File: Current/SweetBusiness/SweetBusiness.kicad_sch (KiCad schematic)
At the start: 42 parts, among them J0 USB, J2 I2C, U0 STM32F411RETx, U1 LDO-3.3, Y1 8MHz

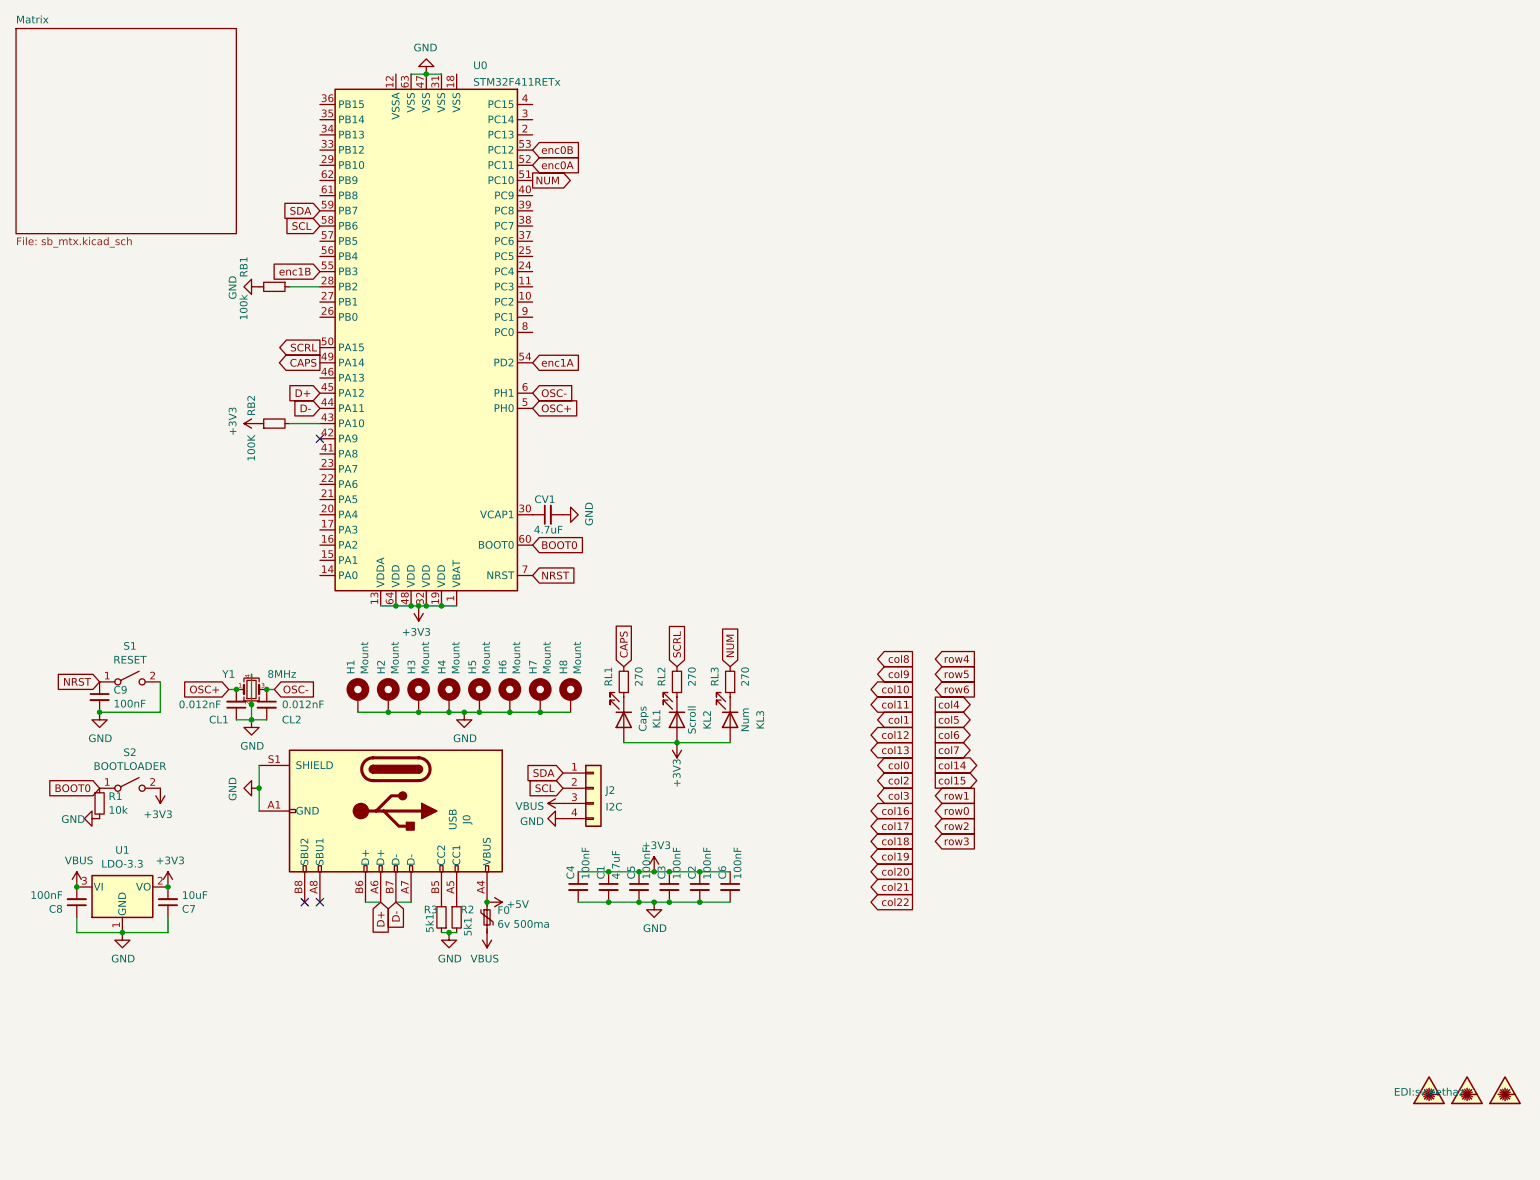
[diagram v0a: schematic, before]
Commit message: Hard Light Micro 5, Borealis, 2T, SB
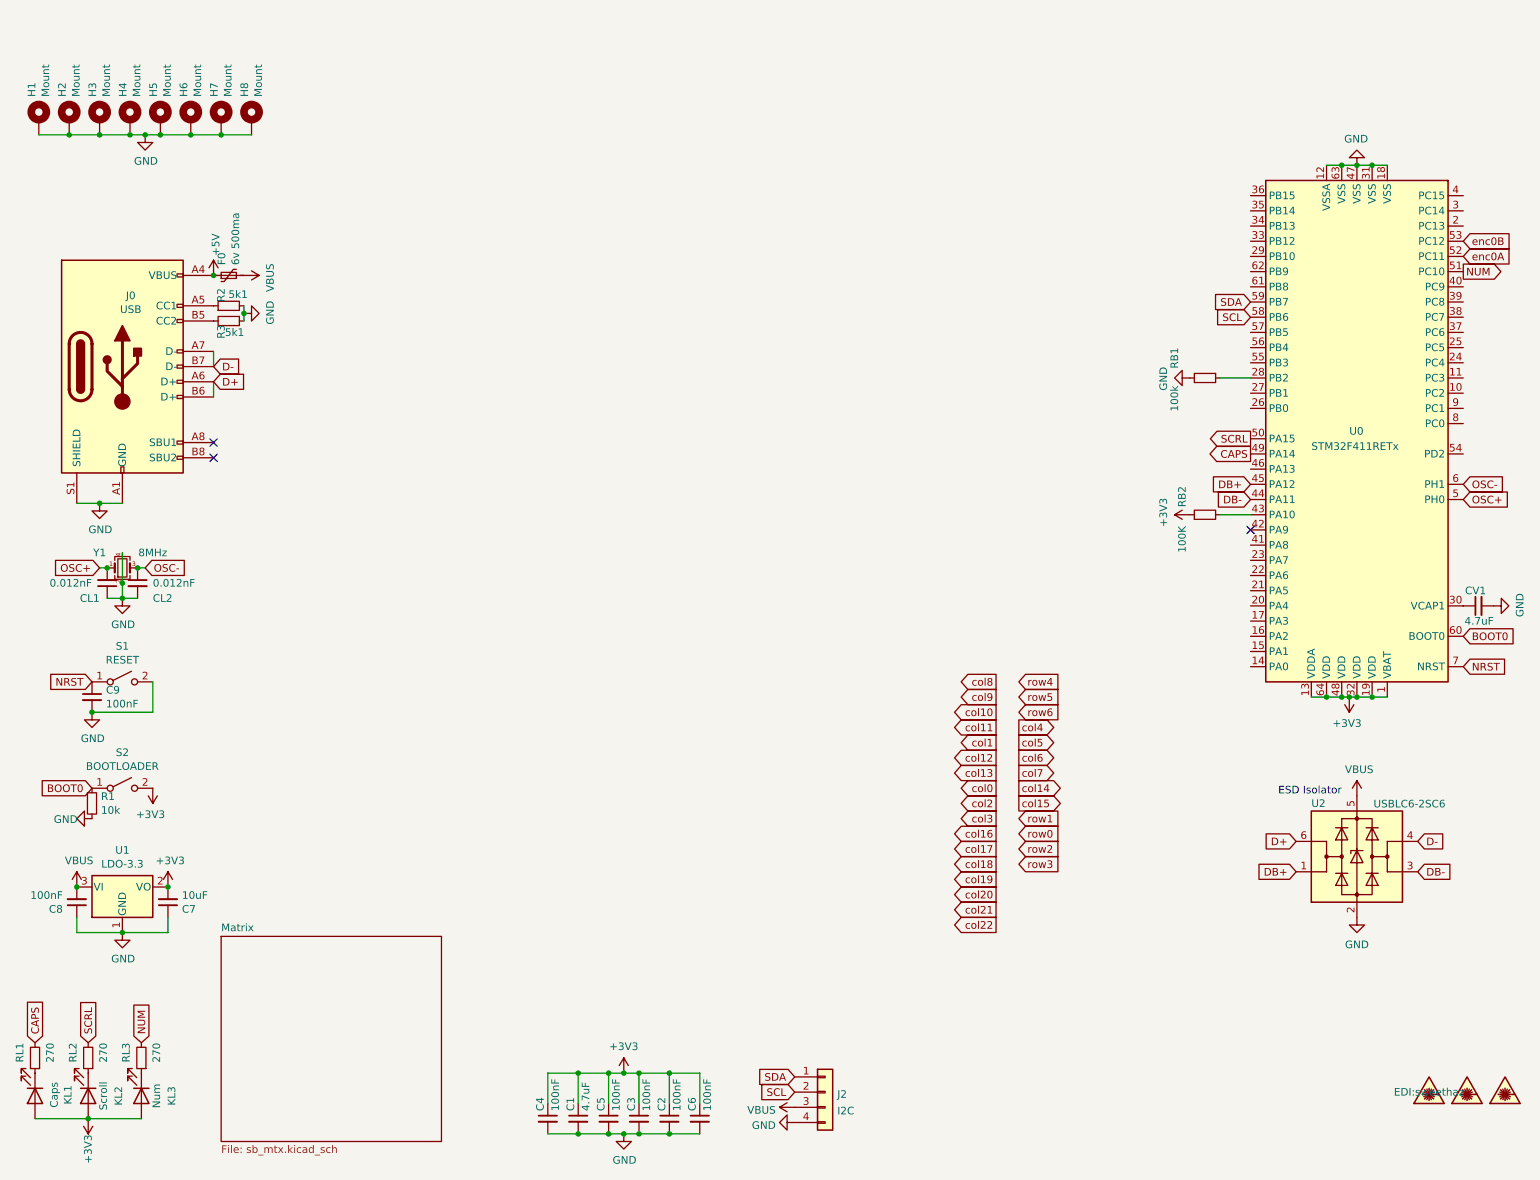
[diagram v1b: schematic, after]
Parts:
- added U2: USBLC6-2SC6, Package_TO_SOT_SMD:SOT-23-6, symbol Power_Protection:USBLC6-2SC6
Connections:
- net D+: now also U2.6 (I/O1); no longer U0.45 (PA12)
- net D-: now also U2.4 (I/O2); no longer U0.44 (PA11)
- net GND: now also U0.12 (VSSA), U0.18 (VSS), U2.2 (GND)
- net VBUS: now also U2.5 (VBUS)
- net enc1A: no longer names the net of U0.54 (PD2)
- net enc1B: no longer names the net of U0.55 (PB3)
- new net DB+: U0.45 (PA12), U2.1 (I/O1)
- new net DB-: U0.44 (PA11), U2.3 (I/O2)
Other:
- note added: "ESD Isolator"
- moved on the sheet: C1, C2, C3, C4, C5, C6, C9, CL1, CL2, CV1, F0, H1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
